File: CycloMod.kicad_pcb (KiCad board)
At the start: 4 copper layers, 22 x 22 mm, 72 parts, among them J1 MICROMOD-2222, U1 10CL010YM164, U2 W25Q128JVS, U3 1.2V, U4 RP2350_60QFN, U5 MIC5504-2.5YMT, Y1 ABM8-272-T3

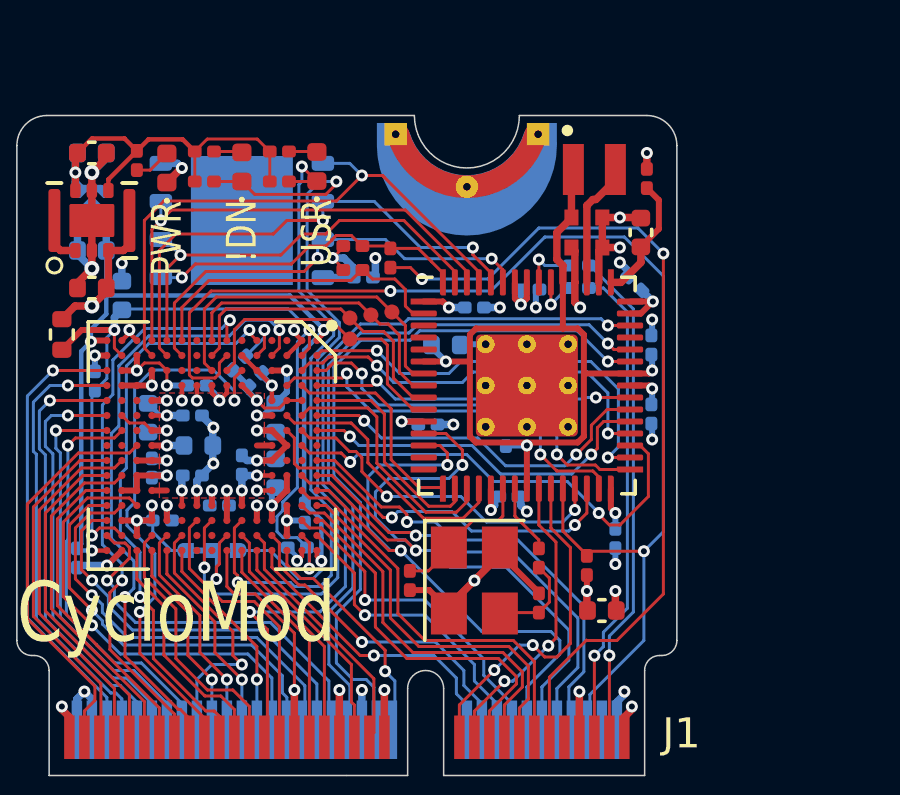
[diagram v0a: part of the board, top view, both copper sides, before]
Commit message: commiting as submitted for build
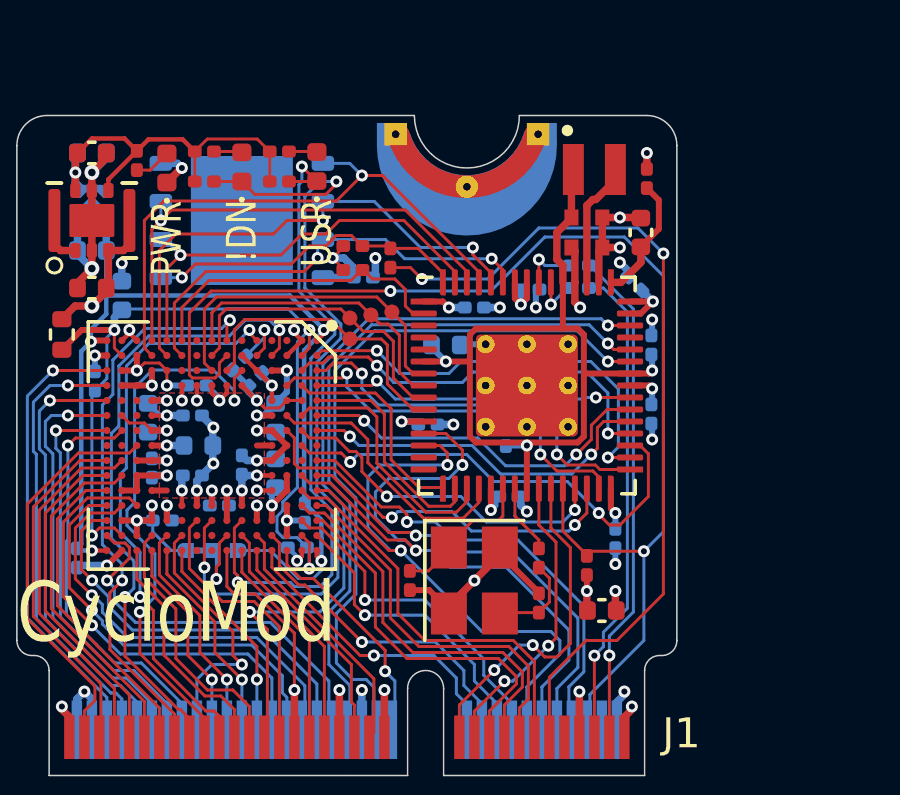
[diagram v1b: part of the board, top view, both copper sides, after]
